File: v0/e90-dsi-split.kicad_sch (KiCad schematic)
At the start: 28 parts, among them J1 3-2328724-1, J2 BM23PF0.8-40DP-0.35V_51_, U1 ICM-42605, U3 LTC3638xMSE

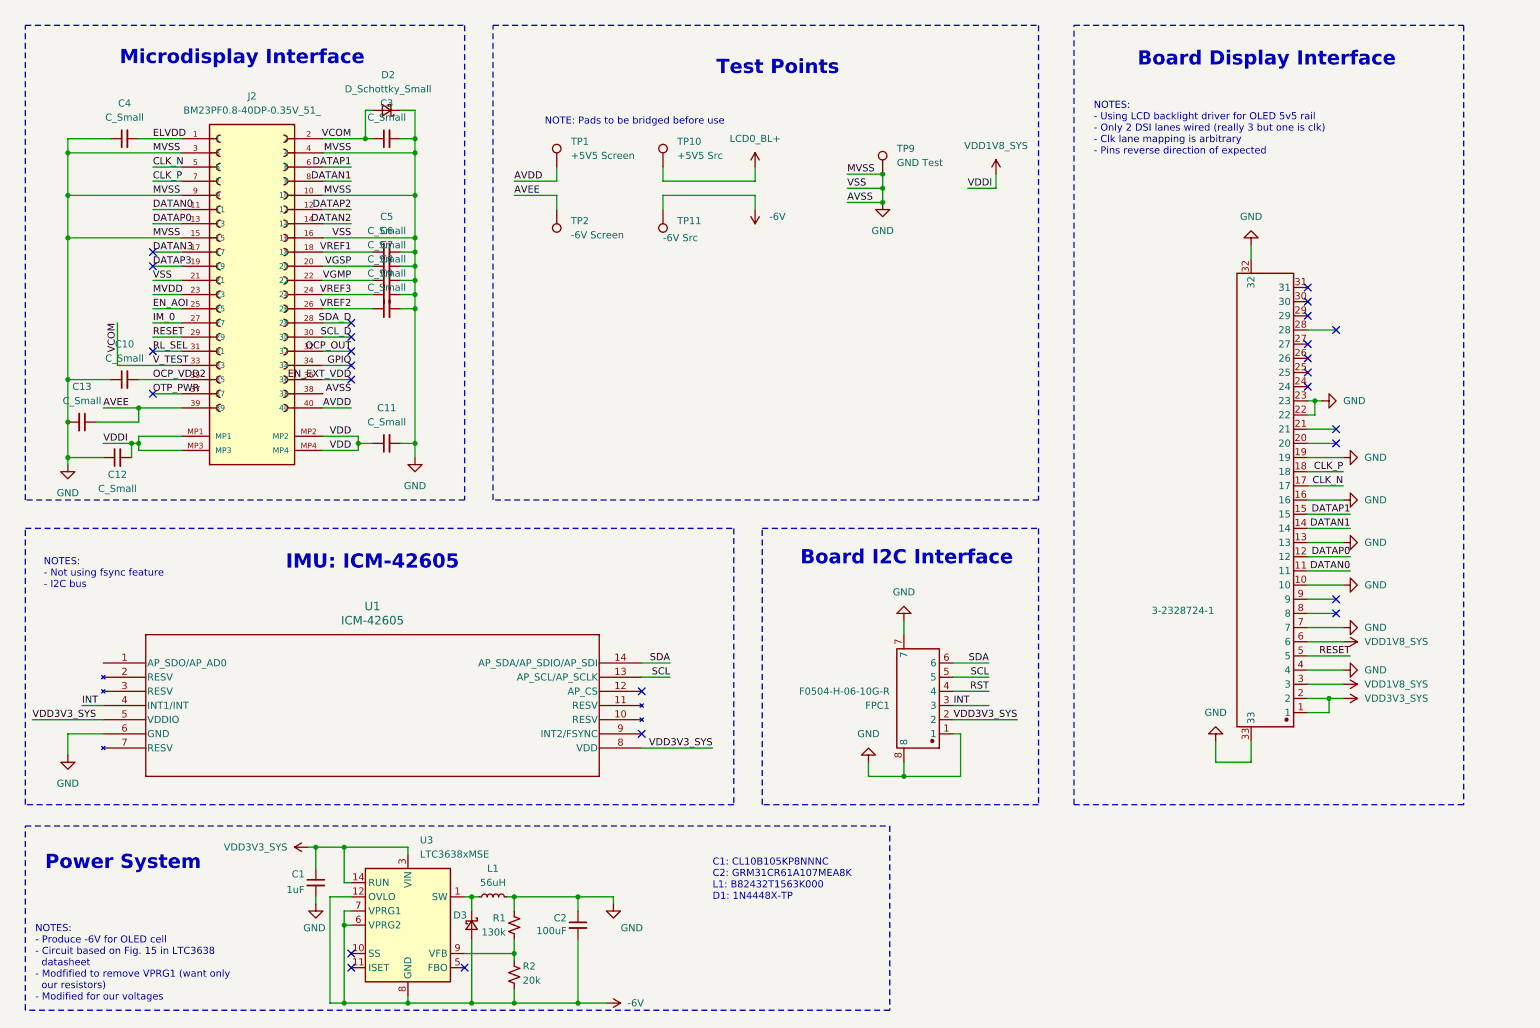
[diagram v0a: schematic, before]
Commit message: v2: continue
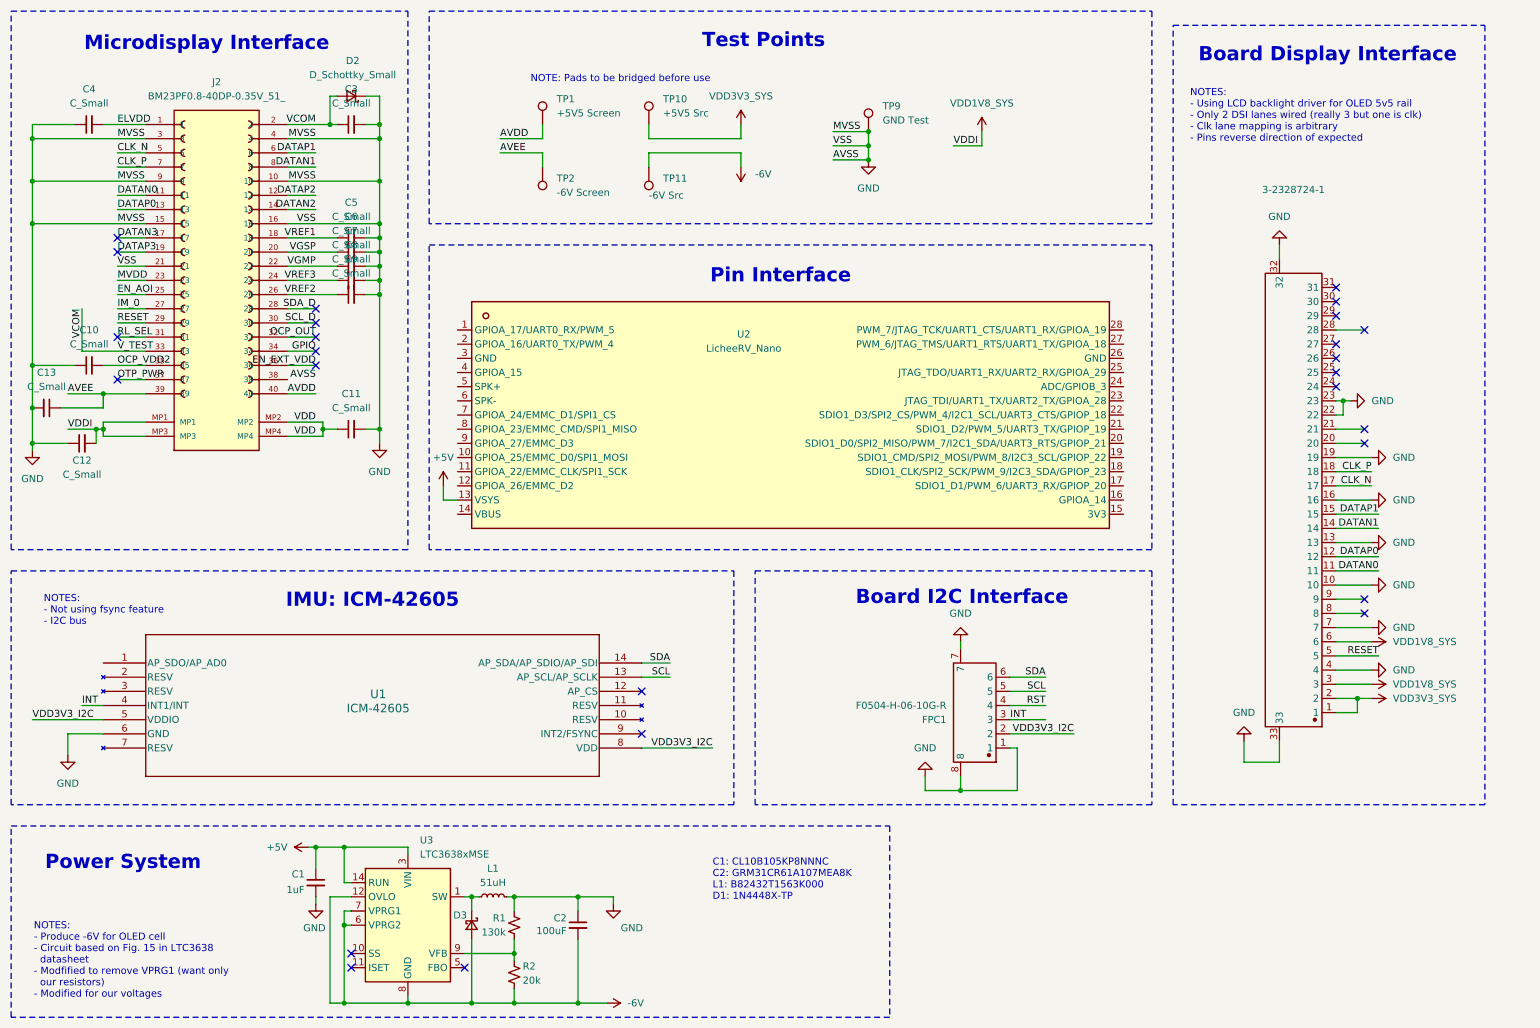
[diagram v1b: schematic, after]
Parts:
- added U2: LicheeRV_Nano, Module:LicheeRV_Nano, symbol Core_moudle:LicheeRV_Nano
- C10, C11, C12, C13, C3, C4, C5, C6, C7, C8, C9: footprint (none) -> Capacitor_SMD:C_0603_1608Metric
- D2, D3: footprint (none) -> Diode_SMD:D_SOD-123
- L1: value 56uH -> 51uH
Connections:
- net LCD0_BL+ is gone; now on net VDD3V3_SYS: TP10.1
- net VDD3V3_SYS: no longer C1.1, FPC1.2, U1.5 (VDDIO), U1.8 (VDD), U3.14 (RUN), U3.3 (VIN)
- new net +5V: C1.1, U2.13 (VSYS), U3.14 (RUN), U3.3 (VIN)
- new net VDD3V3_I2C: FPC1.2, U1.5 (VDDIO), U1.8 (VDD)
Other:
- note added: "Pin Interface"
- moved on the sheet: C10, C11, C12, C13, C3, C4, C5, C6, C7, C8, C9, D2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
